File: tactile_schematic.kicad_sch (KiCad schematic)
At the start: 37 parts, among them IC1 CY8C4145PVI-PS431, J1 Conn_01x02, J2 Conn_01x04, J3 Conn_01x04, J4 Conn_01x02

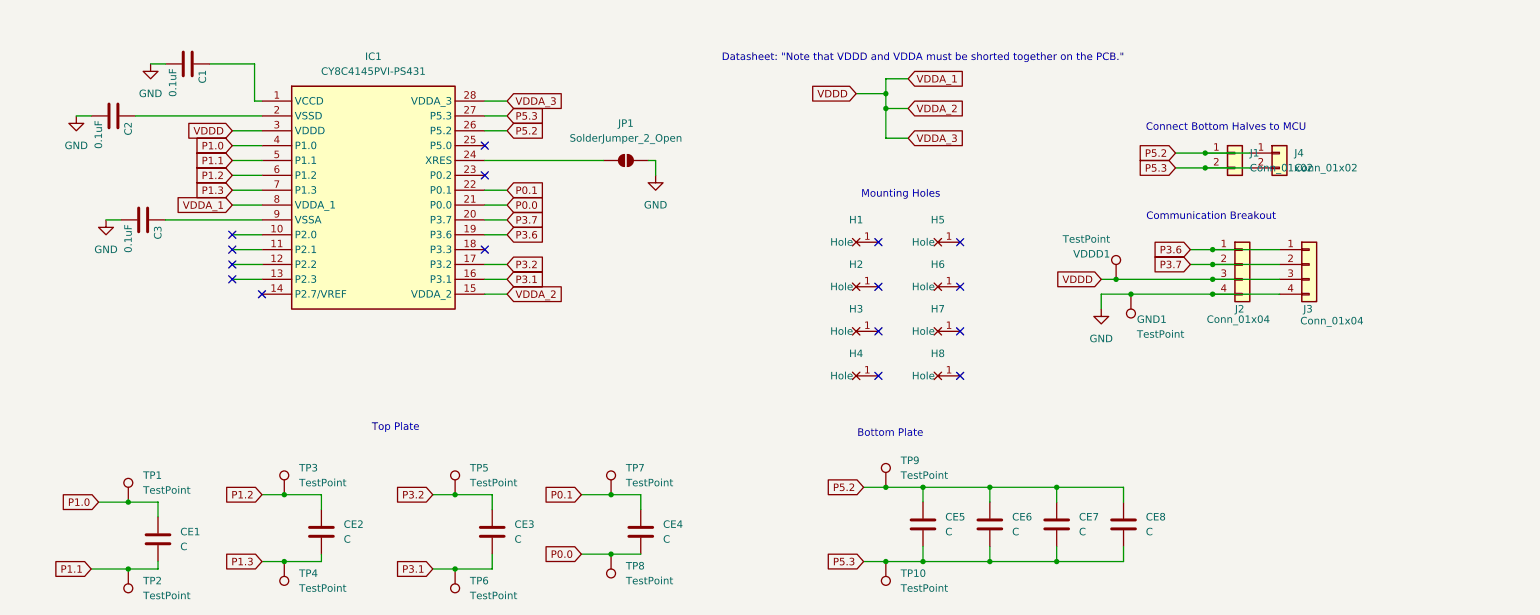
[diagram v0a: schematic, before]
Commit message: many changes
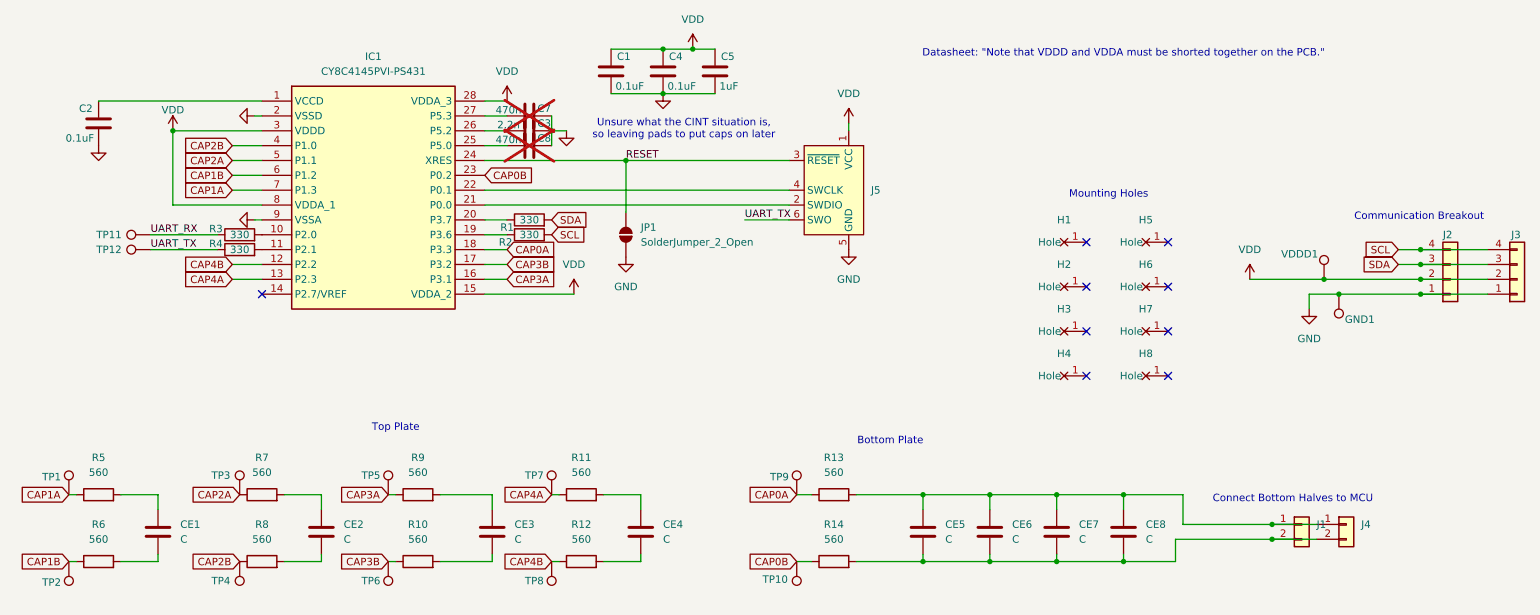
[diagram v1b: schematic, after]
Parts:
- removed C3: 0.1uF, Capacitor_SMD:C_0603_1608Metric_Pad1.08x0.95mm_HandSolder, symbol ECE445L:C
- added C3: 2.2n, Capacitor_SMD:C_0603_1608Metric_Pad1.08x0.95mm_HandSolder, symbol Device:C
- added C4: 0.1uF, Capacitor_SMD:C_0603_1608Metric_Pad1.08x0.95mm_HandSolder, symbol ECE445L:C
- added C5: 1uF, Capacitor_SMD:C_0603_1608Metric_Pad1.08x0.95mm_HandSolder, symbol ECE445L:C
- added C7, C8: 470n, Capacitor_SMD:C_0603_1608Metric_Pad1.08x0.95mm_HandSolder, symbol Device:C
- added J5: Conn_ARM_SWD_TagConnect_TC2030-NL, Connector:Tag-Connect_TC2030-IDC-NL_2x03_P1.27mm_Vertical, symbol Connector:Conn_ARM_SWD_TagConnect_TC2030-NL
- added R1, R2, R3, R4: 330, Resistor_SMD:R_0603_1608Metric_Pad0.98x0.95mm_HandSolder, symbol Device:R
- added R10, R11, R12, R13, R14, R5, R6, R7, R8, R9: 560, Resistor_SMD:R_0603_1608Metric_Pad0.98x0.95mm_HandSolder, symbol Device:R
- added TP11, TP12: TestPoint, TestPoint:TestPoint_THTPad_D1.0mm_Drill0.5mm, symbol Connector:TestPoint
- J2: footprint Connector_PinHeader_2.00mm:PinHeader_1x04_P2.00mm_Vertical -> Connector_PinHeader_1.27mm:PinHeader_1x04_P1.27mm_Vertical
- J3: footprint Connector_JST:JST_SH_SM03B-SRSS-TB_1x03-1MP_P1.00mm_Horizontal -> Connector_JST:JST_SH_SM04B-SRSS-TB_1x04-1MP_P1.00mm_Horizontal
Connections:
- net GND: now also IC1.2 (VSSD), IC1.9 (VSSA), J2.1 (Pin_1), J3.1 (Pin_1), JP1.1 (A), C3.2, C4.2, C5.2, C7.2, C8.2, J5.5 (GND); no longer J2.4 (Pin_4), J3.4 (Pin_4), JP1.2 (B)
- net at IC1.1 (VCCD): now also C2.1; no longer C1.1
- net RESET: now reaches IC1.24 (XRES)
- net RESET: now also JP1.2 (B), J5.3 (~{RESET}); no longer JP1.1 (A)
- net at IC1.10 (P2.0): now also R3.2
- net at IC1.11 (P2.1): now also R4.2
- net CAP4B: now reaches IC1.12 (P2.2)
- net CAP4B: now also TP8.1, R12.1
- net CAP4A: now reaches IC1.13 (P2.3)
- net CAP4A: now also TP7.1, R11.1
- net CAP0A: now reaches IC1.18 (P3.3)
- net CAP0A: now also TP9.1, R13.1
- net CAP0B: now reaches IC1.23 (P0.2)
- net CAP0B: now also TP10.1, R14.1
- net at IC1.25 (P5.0): now also C8.1
- removed net P0.0: CE4.2, IC1.21 (P0.0), TP8.1
- removed net P0.1: CE4.1, IC1.22 (P0.1), TP7.1
- removed net P1.0: CE1.1, IC1.4 (P1.0), TP1.1
- removed net P1.1: CE1.2, IC1.5 (P1.1), TP2.1
- removed net P1.2: CE2.1, IC1.6 (P1.2), TP3.1
- removed net P1.3: CE2.2, IC1.7 (P1.3), TP4.1
- removed net P3.1: CE3.2, IC1.16 (P3.1), TP6.1
- removed net P3.2: CE3.1, IC1.17 (P3.2), TP5.1
- removed net P3.6: IC1.19 (P3.6), J2.1 (Pin_1), J3.1 (Pin_1)
- net P3.7 renamed VDD
- net VDD: now also C1.1, IC1.15 (VDDA_2), IC1.28 (VDDA_3), IC1.3 (VDDD), IC1.8 (VDDA_1), VDDD1.1, C4.1, C5.1, J5.1 (VCC); no longer IC1.20 (P3.7)
- net P5.2: no longer names the net of CE5.1, CE6.1, CE7.1, CE8.1, J1.1 (Pin_1), J4.1 (Pin_1)
- net P5.2: now also R13.2; no longer IC1.26 (P5.2), TP9.1
- net P5.3: no longer names the net of CE5.2, CE6.2, CE7.2, CE8.2, J1.2 (Pin_2), J4.2 (Pin_2)
- net P5.3: now also R14.2; no longer IC1.27 (P5.3), TP10.1
- removed net VDDA_1: IC1.15 (VDDA_2), IC1.28 (VDDA_3), IC1.3 (VDDD), IC1.8 (VDDA_1), J2.3 (Pin_3), J3.3 (Pin_3), VDDD1.1
- new net: C7.1, IC1.27 (P5.3)
- new net: IC1.20 (P3.7), R1.1
- new net: CE1.1, R5.2
- new net: CE1.2, R6.2
- new net: CE4.2, R12.2
- new net: C3.1, IC1.26 (P5.2)
- new net: CE3.2, R10.2
- new net: IC1.21 (P0.0), J5.2 (SWDIO)
- new net: IC1.22 (P0.1), J5.4 (SWCLK)
- new net: CE2.2, R8.2
- new net: CE4.1, R11.2
- new net: CE3.1, R9.2
- new net: IC1.19 (P3.6), R2.1
- new net: CE2.1, R7.2
- new net CAP1A: IC1.7 (P1.3), R5.1, TP1.1
- new net CAP1B: IC1.6 (P1.2), R6.1, TP2.1
- new net CAP2A: IC1.5 (P1.1), R7.1, TP3.1
- new net CAP2B: IC1.4 (P1.0), R8.1, TP4.1
- new net CAP3A: IC1.16 (P3.1), R9.1, TP5.1
- new net CAP3B: IC1.17 (P3.2), R10.1, TP6.1
- new net SCL: J2.4 (Pin_4), J3.4 (Pin_4), R2.2
- new net SDA: J2.3 (Pin_3), J3.3 (Pin_3), R1.2
- new net UART_RX: R3.1, TP11.1
- new net UART_TX: J5.6 (SWO), R4.1, TP12.1
- no-connect marks 16 -> 9
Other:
- note added: "Unsure what the CINT situation is, so leaving pads to put caps on later"
- moved on the sheet: C1, CE1, CE5, CE6, CE7, CE8, GND1, H1, H2, H3, H4, H5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
